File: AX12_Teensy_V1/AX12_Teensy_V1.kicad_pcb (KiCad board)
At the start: 2 copper layers, 60.7 x 41.4 mm, 24 parts, among them IC1 TEENSY3.2, J1 uart, J10 Conn_CAN, J2 AX12, J3 AX12, J4 AX12, J5 AX12, J8 12VP, J9 Conn_CAN, U1 SN65HVD232

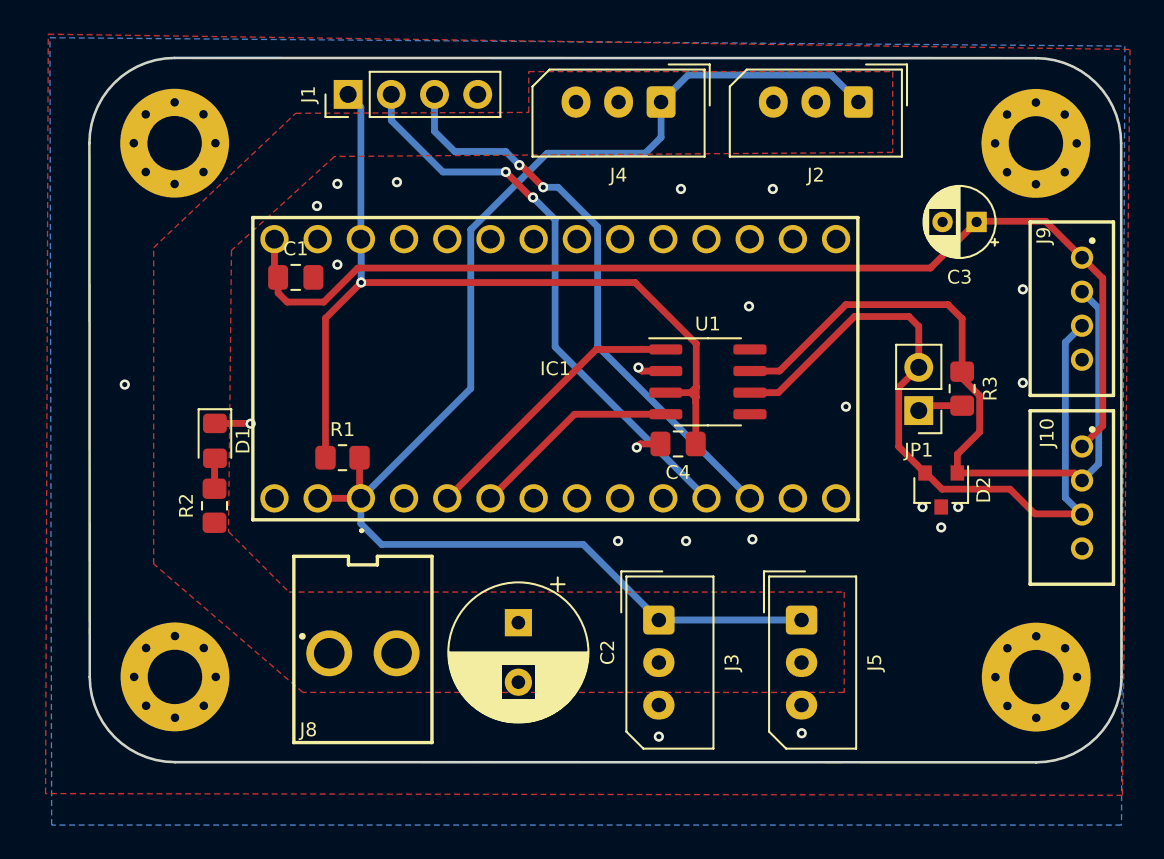
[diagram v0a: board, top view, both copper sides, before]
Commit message: change connector and some final touch
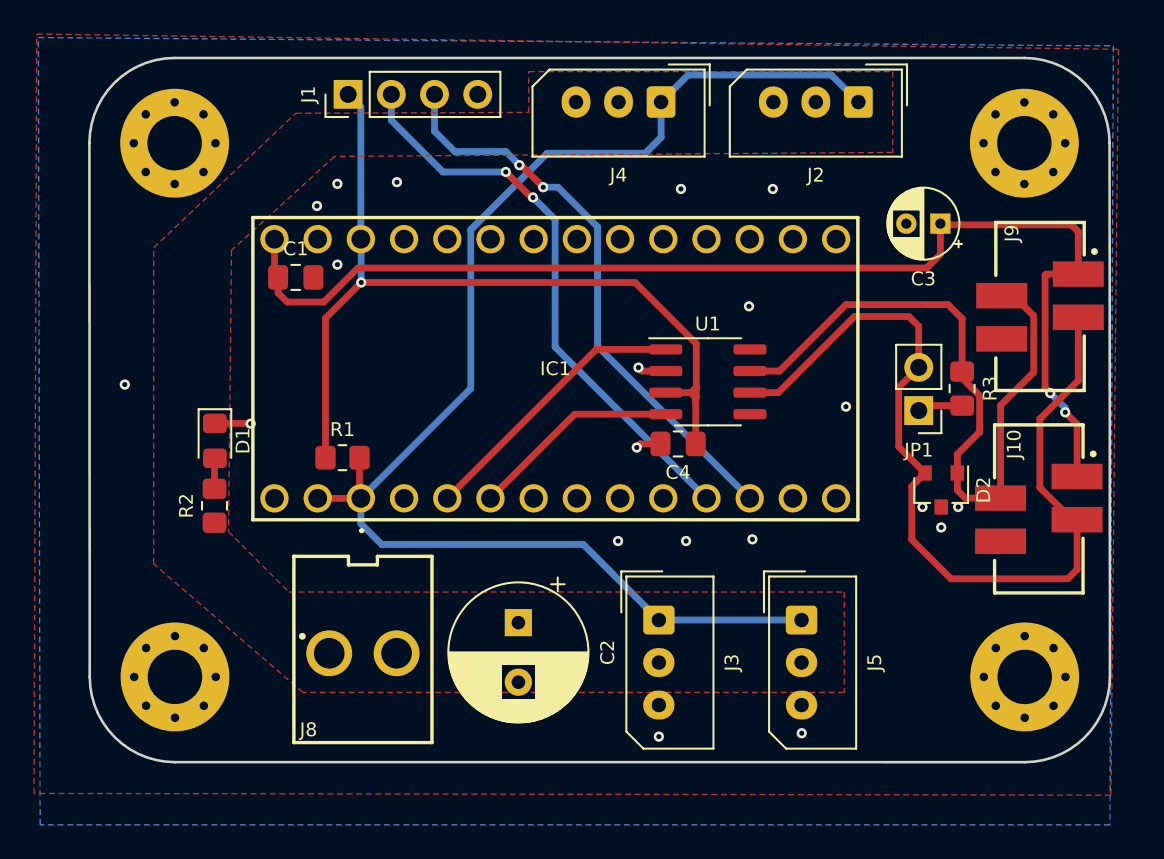
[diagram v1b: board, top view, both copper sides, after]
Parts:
- J10, J9: footprint AREA_lib_Connector:Wuerth_2mm_4pin_62000411622 -> AREA_lib_Connector:690367290476
- moved C3 2.13 mm to (153.7, 54.2)
- moved J10 2.05 mm to (159.4, 71.0)
- moved J9 1.87 mm to (159.5, 59.1)
- moved H3 0.68 mm to (158.6, 49.5)
- moved H2 0.68 mm to (158.6, 80.9)
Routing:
- net /CANL: track 43.9 -> 53.8 mm
- net +5V: track 65.7 -> 70.8 mm, vias 0 -> 2
- net /CANH: track 43.9 -> 42.1 mm
- net GND: vias 22 -> 20
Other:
- board size 60.7 x 41.4 mm -> 60 x 41.4 mm
